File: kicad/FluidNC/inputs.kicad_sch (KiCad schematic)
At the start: 118 parts, among them J10 Conn_01x02_Socket, J11 Conn_01x02_Socket, J12 Conn_01x02_Socket, J13 Conn_01x02_Socket, J14 Conn_01x02_Socket, J15 Conn_01x02_Socket, J16 Conn_01x12_Socket, SW10 Macro 2, SW11 Macro 3, SW12 Resume, SW13 Pause, SW9 Macro 1, U21 LTV-847, U22 74HC14, U23 74HC14, U24 LTV-847, U25 LTV-847

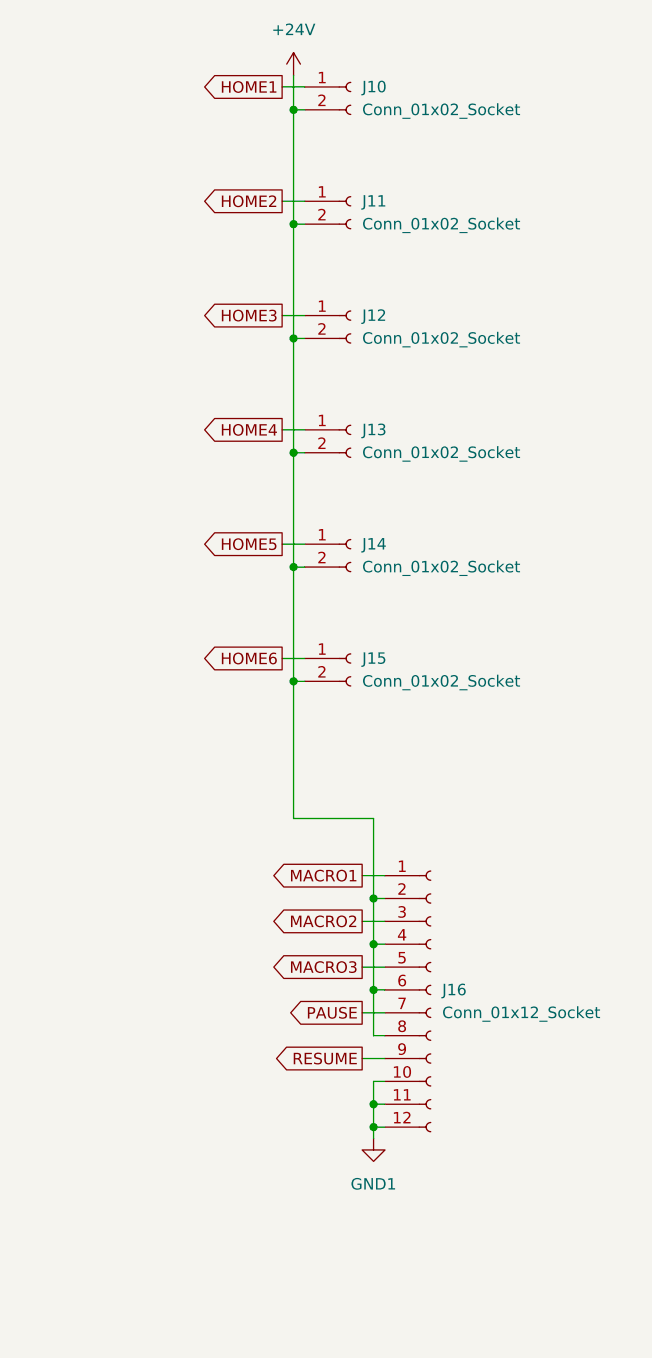
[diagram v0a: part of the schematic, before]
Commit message: Add V2R1
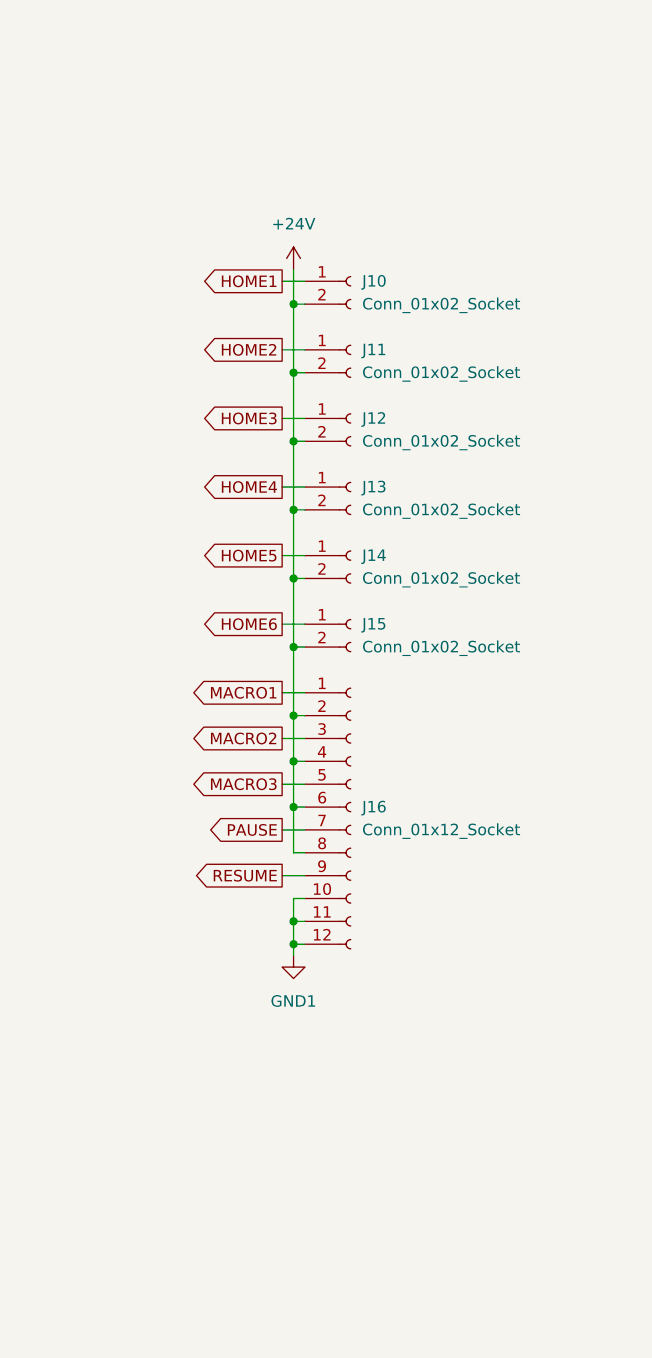
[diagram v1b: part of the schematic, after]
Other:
- moved on the sheet: J10, J11, J12, J13, J14, J15, J16
